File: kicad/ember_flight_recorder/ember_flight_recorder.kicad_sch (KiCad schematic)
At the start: 18 parts, among them Q3 FS8205A, Q4 AO3401A, U2 DW01A, U3 MCP1700x-330xxTT, U4 module_mpu6050, U5 module_bme280, U6 ESP32-C3_SUPERMINI_SMD

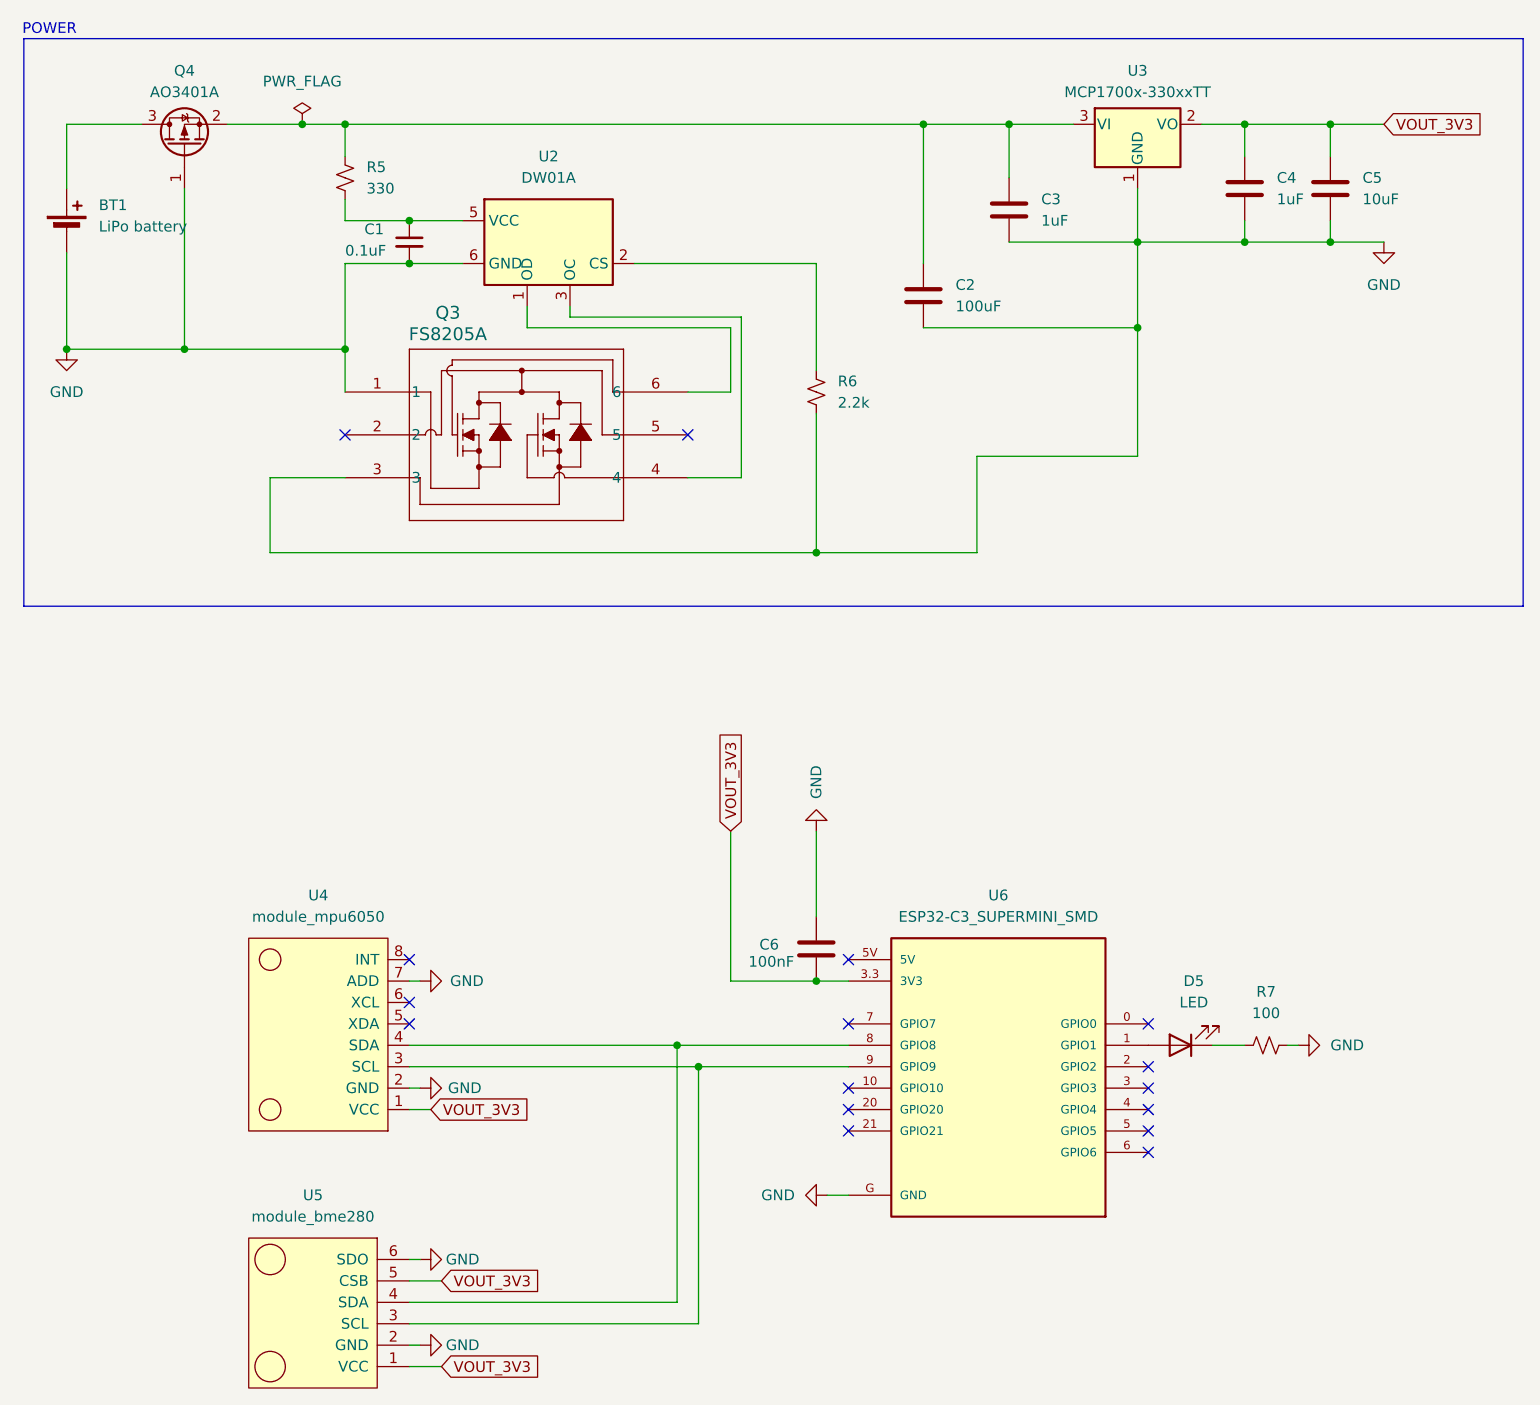
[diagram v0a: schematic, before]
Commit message: flight recorder rev1
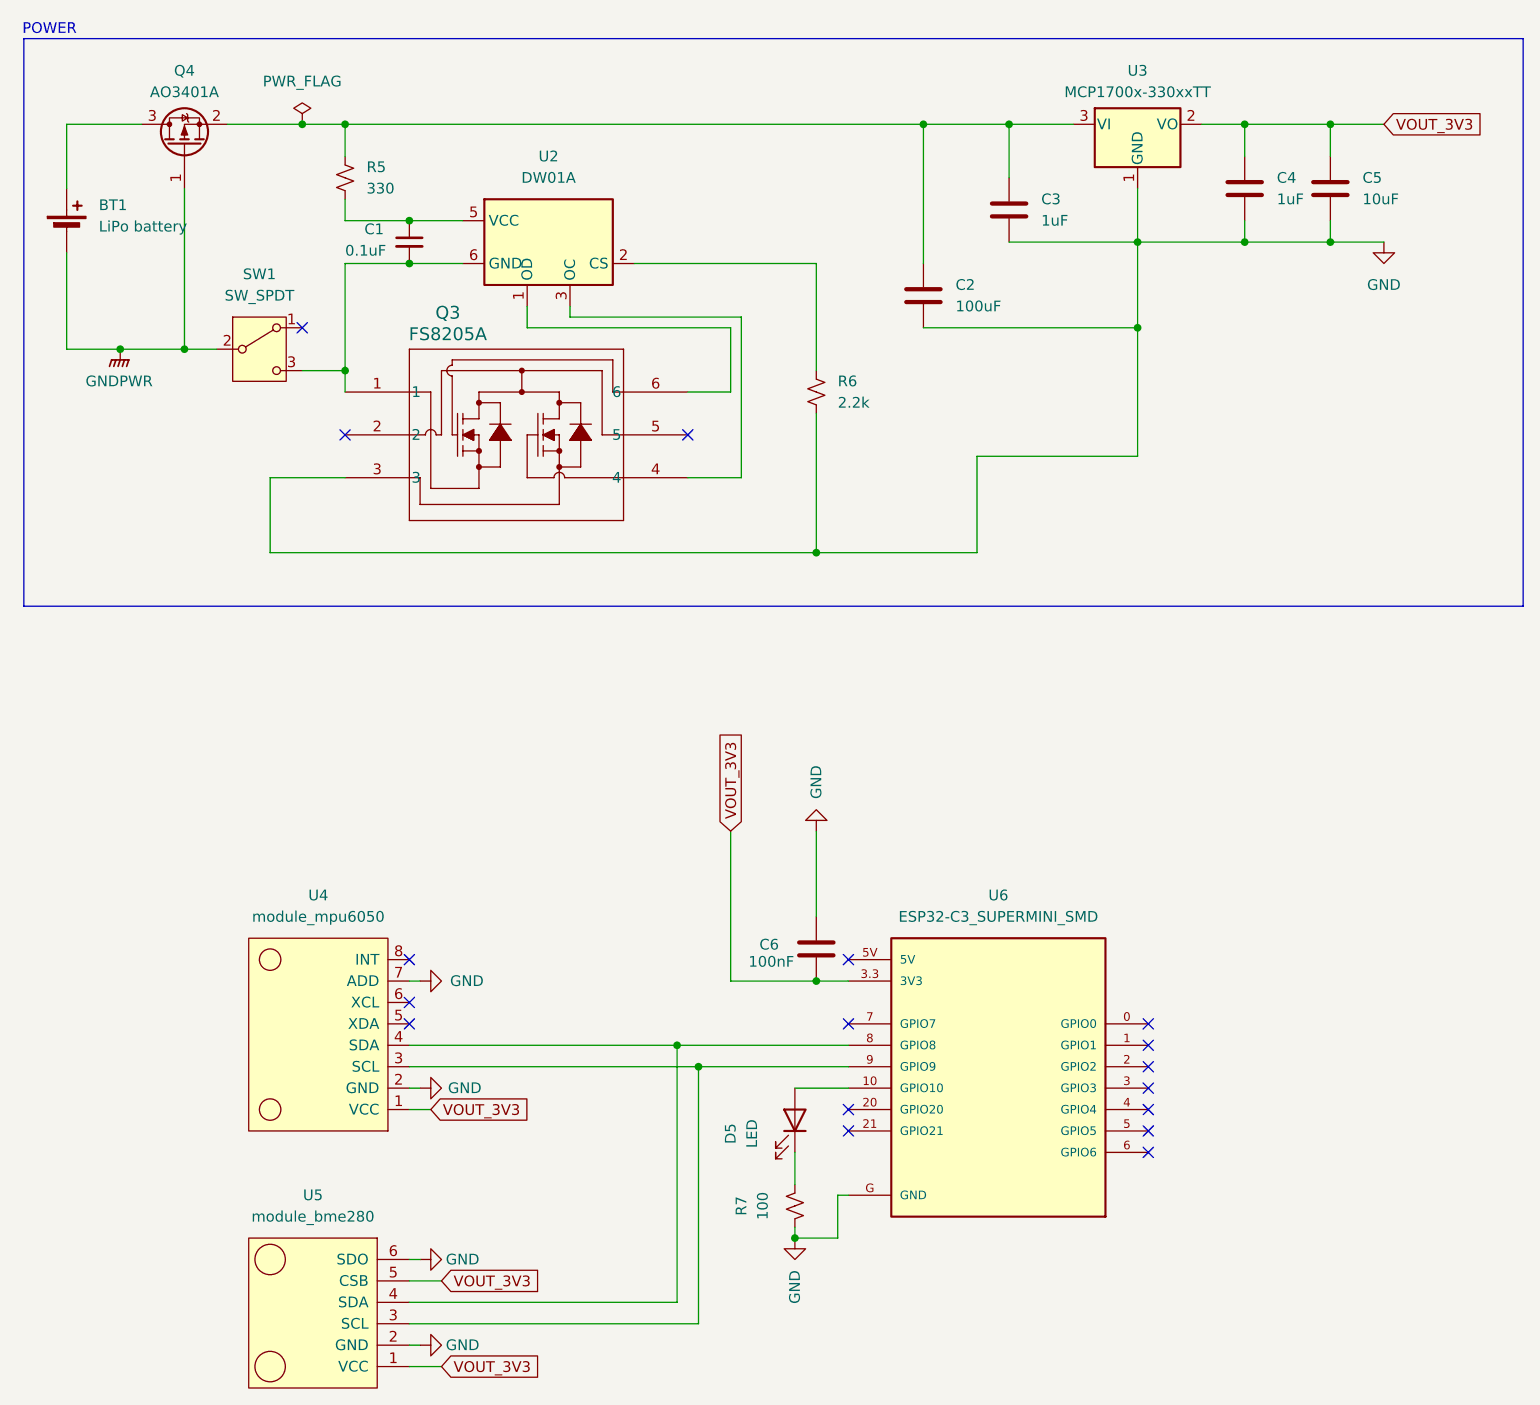
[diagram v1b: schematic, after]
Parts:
- added SW1: SW_SPDT, Button_Switch_THT:SW_Slide-03_Wuerth-WS-SLTV_10x2.5x6.4_P2.54mm, symbol Switch:SW_SPDT
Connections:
- net GND: no longer BT1.2 (-), C1.2, Q3.1, Q4.1 (G), U2.6 (GND)
- net at U6.1 (GPIO1): no longer D5.2 (A)
- net at U6.10 (GPIO10): now also D5.2 (A)
- new net: C1.2, Q3.1, SW1.3 (C), U2.6 (GND)
- new net GNDPWR: BT1.2 (-), Q4.1 (G), SW1.2 (B)
- no-connect marks 16 -> 17
